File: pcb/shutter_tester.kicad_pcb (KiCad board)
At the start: 2 copper layers, 53 x 42 mm, 17 parts, among them J1 Conn_01x04, Q1 MMBTA13LT3G, U1 LM393

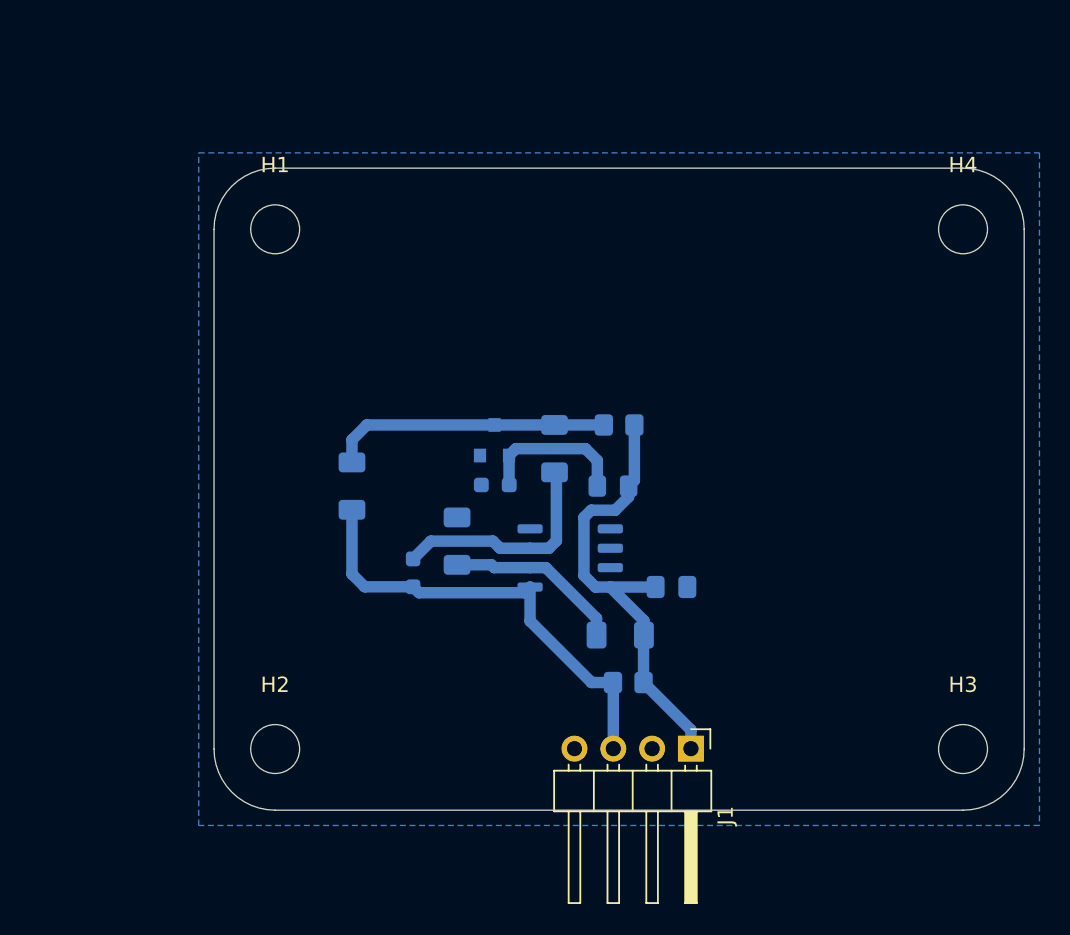
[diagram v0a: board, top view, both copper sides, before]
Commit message: getting to rev b layout
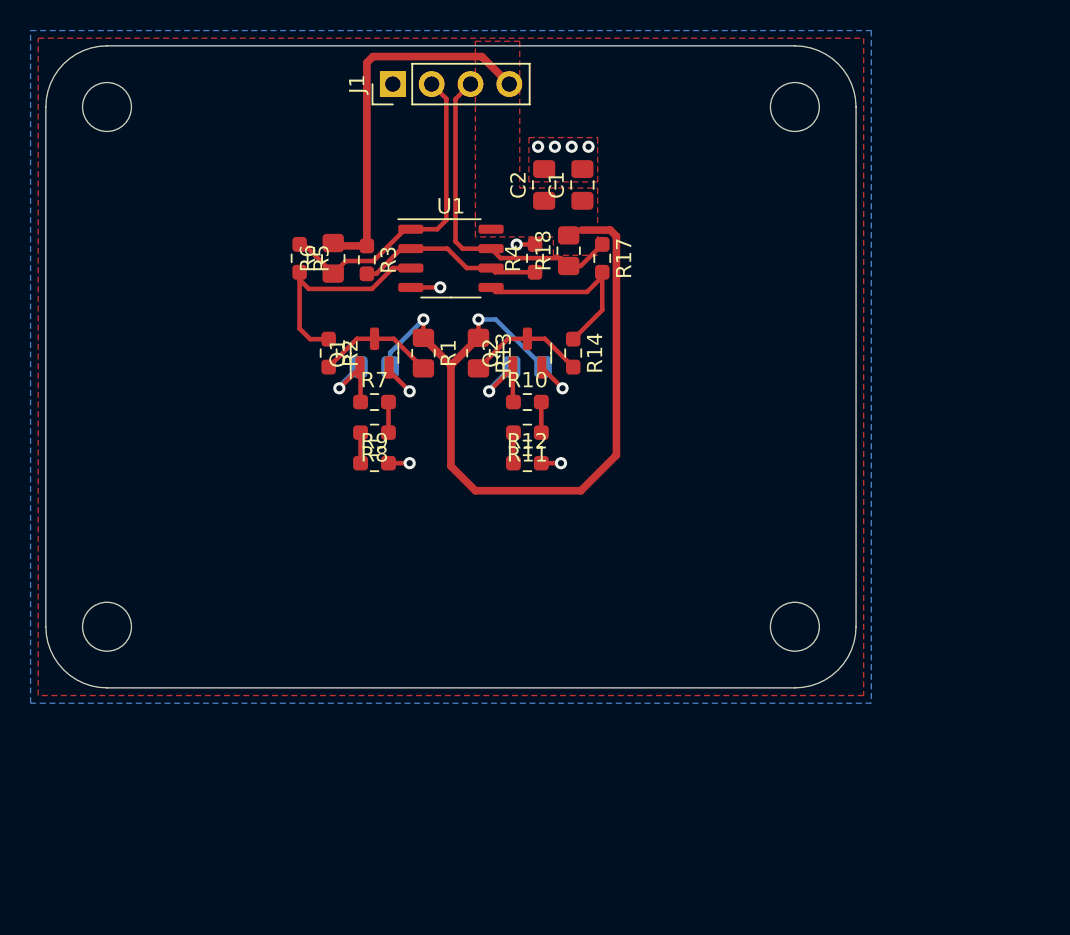
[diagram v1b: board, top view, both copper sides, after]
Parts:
- removed JP1: Comparitor Bypass, Resistor_SMD:R_1206_3216Metric_Pad1.30x1.75mm_HandSolder
- added C2: 1u, Capacitor_SMD:C_0805_2012Metric_Pad1.18x1.45mm_HandSolder, F.Cu at (152.6, 102.1)
- added D2: LED, LED_SMD:LED_0805_2012Metric_Pad1.15x1.40mm_HandSolder, B.Cu at (151.5, 114.0)
- added Q2: MMBTA13LT3G, Package_TO_SOT_SMD:SOT-23, F.Cu at (151.5, 113.1)
- added R10: 4.7M, Resistor_SMD:R_0603_1608Metric_Pad0.98x0.95mm_HandSolder, F.Cu at (151.5, 116.3)
- added R11: 4.7M, Resistor_SMD:R_0603_1608Metric_Pad0.98x0.95mm_HandSolder, F.Cu at (151.5, 118.3)
- added R12: 4.7M, Resistor_SMD:R_0603_1608Metric_Pad0.98x0.95mm_HandSolder, F.Cu at (151.5, 120.3)
- added R13: 2k, Resistor_SMD:R_0805_2012Metric_Pad1.20x1.40mm_HandSolder, F.Cu at (148.3, 113.1)
- added R14: 10k, Resistor_SMD:R_0603_1608Metric_Pad0.98x0.95mm_HandSolder, F.Cu at (154.5, 113.1)
- added R17: 102k, Resistor_SMD:R_0603_1608Metric_Pad0.98x0.95mm_HandSolder, F.Cu at (156.4, 106.9)
- added R18: 3k, Resistor_SMD:R_0805_2012Metric_Pad1.20x1.40mm_HandSolder, F.Cu at (154.2, 106.4)
- added R8: 4.7M, Resistor_SMD:R_0603_1608Metric_Pad0.98x0.95mm_HandSolder, F.Cu at (141.5, 118.3)
- added R9: 4.7M, Resistor_SMD:R_0603_1608Metric_Pad0.98x0.95mm_HandSolder, F.Cu at (141.5, 120.3)
- C1, Q1, R1, R5, R6, R7, U1: moved to F.Cu
- J1: footprint Connector_PinHeader_2.54mm:PinHeader_1x04_P2.54mm_Horizontal -> Connector_PinHeader_2.54mm:PinHeader_1x04_P2.54mm_Vertical
- R2, R3, R4: footprint Resistor_SMD:R_1206_3216Metric_Pad1.30x1.75mm_HandSolder -> Resistor_SMD:R_0603_1608Metric_Pad0.98x0.95mm_HandSolder; moved to F.Cu
- moved J1 47.6 mm to (142.7, 95.5), turned to 90 degrees
- moved R6 33.8 mm to (138.8, 106.9), turned to 90 degrees
- moved R3 29.6 mm to (141.0, 107.0), turned to -90 degrees
- moved C1 26.9 mm to (155.1, 102.1), turned to 90 degrees
- moved R5 21.9 mm to (136.6, 106.9), turned to -90 degrees
- moved U1 21.1 mm to (146.5, 106.9)
- moved R4 19.2 mm to (152.0, 106.9), turned to 90 degrees
- moved D1 17.4 mm to (141.5, 114.0)
- moved R2 16.0 mm to (138.5, 113.1), turned to -90 degrees
- moved R1 13.6 mm to (144.7, 113.1), turned to -90 degrees
- moved H1 13.6 mm to (124.0, 97.0)
- moved H2 13.6 mm to (124.0, 131.0)
- moved H3 13.6 mm to (169.0, 131.0)
- moved H4 13.6 mm to (169.0, 97.0)
- moved Q1 9.70 mm to (141.5, 113.1)
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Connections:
- J1 pad 1: VCC -> GND
- J1 pad 2: GND -> /OUTPUT_1
- J1 pad 3: /OUTPUT -> /OUTPUT_2
- J1 pad 4: GND -> VCC
- R3 pad 1: Net-(R3-Pad1) -> VCC
- R3 pad 2: VCC -> /Vtrig
- R4 pad 1: GND -> /Vtrig
- R4 pad 2: Net-(R3-Pad1) -> GND
- R5 pad 1: /OUTPUT -> /OUTPUT_1
- R6 pad 1: /OUTPUT -> /OUTPUT_1
- R7 pad 2: GND -> Net-(R7-Pad2)
- U1 pad 1: /OUTPUT -> /OUTPUT_1
- U1 pad 2: Net-(R3-Pad1) -> /Vtrig
- U1 pad 5: GND -> Net-(U1-Pad5)
- U1 pad 6: GND -> /Vtrig
- U1 pad 7: GND -> /OUTPUT_2
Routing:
- net VCC: track 29.9 -> 77.3 mm, vias 0 -> 2
- net /OUTPUT: track 30.2 -> 0.00 mm
- net /OUTPUT_2: track 0.00 -> 21.6 mm
- net /OUTPUT_1: track 0.00 -> 21.1 mm
- net Net-(U1-Pad5): track 0.00 -> 13.3 mm
- net /Vtrig: track 0.00 -> 12.3 mm
- net Net-(R3-Pad1): track 11.7 -> 0.00 mm
- net Net-(Q1-Pad3): track 18.4 -> 7.77 mm
- net GND: track 0.00 -> 9.85 mm, vias 0 -> 10
- net Net-(Q2-Pad3): track 0.00 -> 7.77 mm
- net Net-(D2-Pad2): track 0.00 -> 6.63 mm, vias 0 -> 1
- net Net-(D1-Pad2): track 9.89 -> 6.06 mm, vias 0 -> 1
- net Net-(R8-Pad2): track 0.00 -> 2.00 mm
- net Net-(R7-Pad2): track 0.00 -> 2.00 mm
- net Net-(R11-Pad2): track 0.00 -> 2.00 mm
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- added copper zone on F.Cu, net (none)
- added copper zone on F.Cu, net GND
- added copper zone on F.Cu, net VCC
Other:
- board text added: "Shutter Boundry"
